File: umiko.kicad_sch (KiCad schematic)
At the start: 396 parts, among them J1 USB_C_Receptacle_USB2.0, J2 USB_C_Receptacle_USB2.0, SW1 SWITCH, SW2 SWITCH, U1 USBLC6-2P6, U10 TLV75533PDQNR, U11 RP2040, U12 TRRS, U2 TLV75533PDQNR, U3 W25Q128JVPIQ, U4 TRRS, U5 SN74LVC1T45DRL, U6 W25Q128JVPIQ, U7 RP2040, U8 SN74LVC1T45DRL, U9 USBLC6-2P6, Y1 12MHz, Y2 12MHz

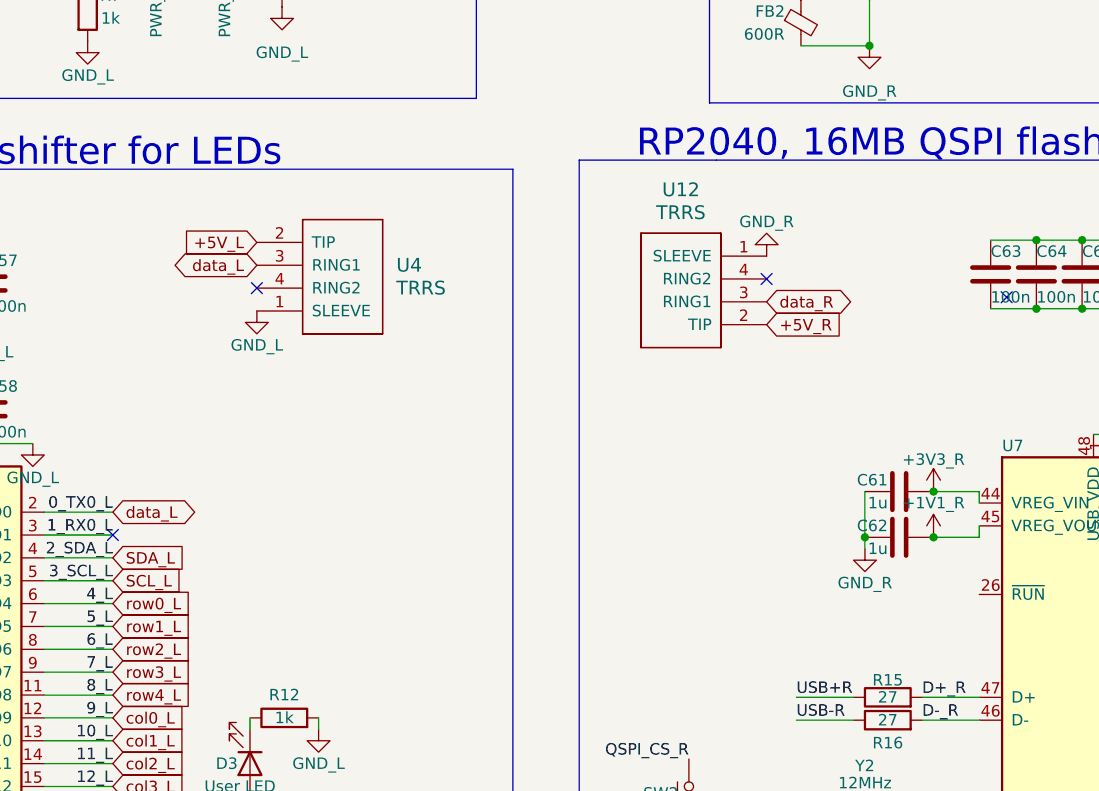
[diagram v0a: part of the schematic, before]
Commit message: Swap inter-half TRRS back to USB-C; rebuild inter-half planks
Reverses the earlier TRRS swap and goes back to USB-C for the inter-half
connection. Two USB-C receptacles (J3 + J4) face each other across the
inter-half gap with a USB-C male-male coupler bridging them.

Schematic:
- Deleted U4/U12 TRRS symbols.
- Added J3 + J4 (Connector:USB_C_Receptacle_USB2.0) at same positions,
  Footprint preset to PCM_0xcb:USB_C_Receptacle_HRO_TYPE-C-31-M-12.
  Used J1 as template; fresh UUIDs for symbol + all 16 pins each.
- User wired up J3/J4: VBUS pins -> +5V_L/+5V_R, GND pins -> GND_L/GND_R,
  data line on D+ (A6/B6) -> data_L/data_R.

PCB:
- Removed the old 2mm flush-to-inner-edge TRRS planks (Y=34-36, X 165-173
  left + X 184-192 right). Restored those inner edges' top corners as
  sharp 90deg transitions to the main board top edge.
- Added new inter-half USB-C planks at the actual J3/J4 body height
  (Y=39.45-50.39, 10.94mm tall = body Y range + 1mm margin each side).
  Each plank protrudes 4mm into the gap from its half's inner edge.
  Outer corners get 0.5mm fillets, inner sides are flush with the inner
  edge vertical. 3.59mm clear gap between planks for the male-male
  coupler to fit.

Scripts: _swap_trrs_to_usbc_schematic.py (the symbol swap) and
_trrs_to_usbc_planks.py (the plank rebuild) saved under scripts/.

Co-Authored-By: Claude Opus 4.7 (1M context) <noreply@anthropic.com>
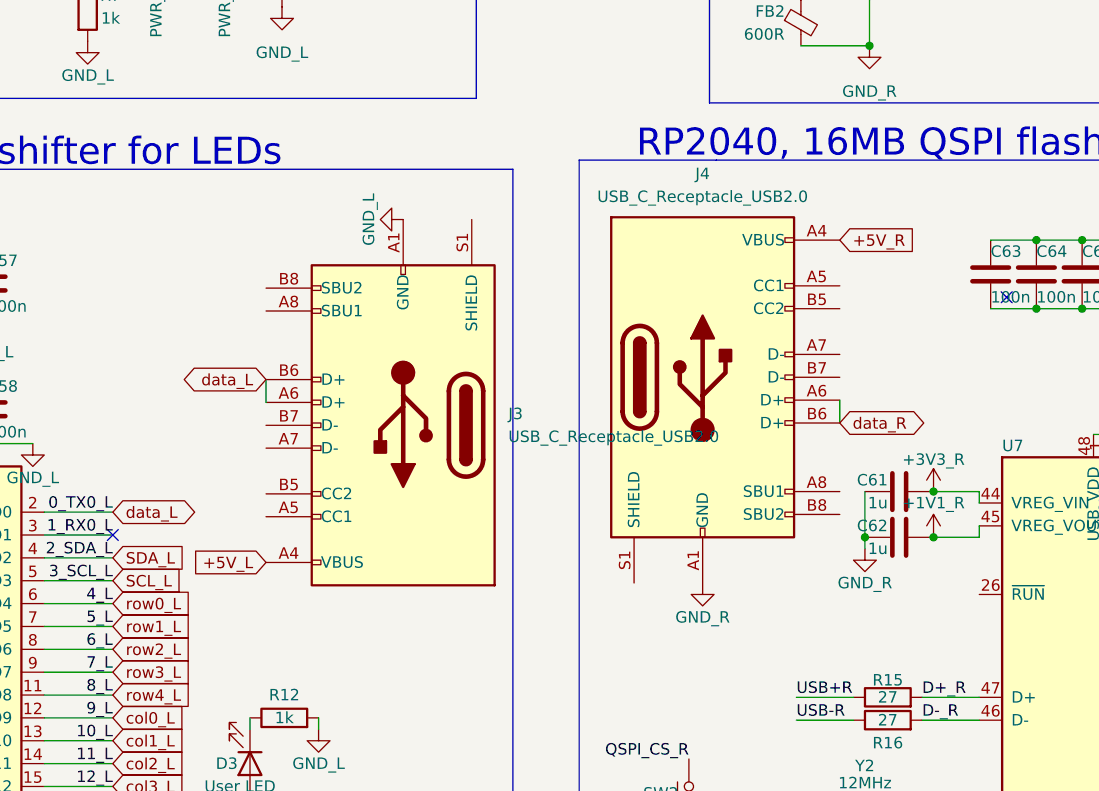
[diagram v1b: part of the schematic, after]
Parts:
- removed U12, U4: TRRS, onigaku:TRRS-PJ-320A, symbol keebio:TRRS
- added J3, J4: USB_C_Receptacle_USB2.0, PCM_0xcb:USB_C_Receptacle_HRO_TYPE-C-31-M-12, symbol Connector:USB_C_Receptacle_USB2.0
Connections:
- net +5V_L: now also J3.A4 (VBUS), J3.A9 (VBUS), J3.B4 (VBUS), J3.B9 (VBUS)
- net +5V_R: now also J4.A4 (VBUS), J4.A9 (VBUS), J4.B4 (VBUS), J4.B9 (VBUS)
- net GND_L: now also J3.A1 (GND), J3.A12 (GND), J3.B1 (GND), J3.B12 (GND)
- net GND_R: now also J4.A1 (GND), J4.A12 (GND), J4.B1 (GND), J4.B12 (GND)
- net data_L: now also J3.A6 (D+), J3.B6 (D+)
- net data_R: now also J4.A6 (D+), J4.B6 (D+)
- no-connect marks 33 -> 31
